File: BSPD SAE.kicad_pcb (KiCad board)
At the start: 2 copper layers, 70 x 70 mm, 66 parts, among them J1 430450412, J2 436500215, K1 G5Q-1A-EU DC12, Q1 MMBT3904, Q2 2N7002K, Q3 MMBT3904, U1 LTC6994xS6-2, U2 TPS7A2501DRVR, U3 TLV1824, U4 TLV1824

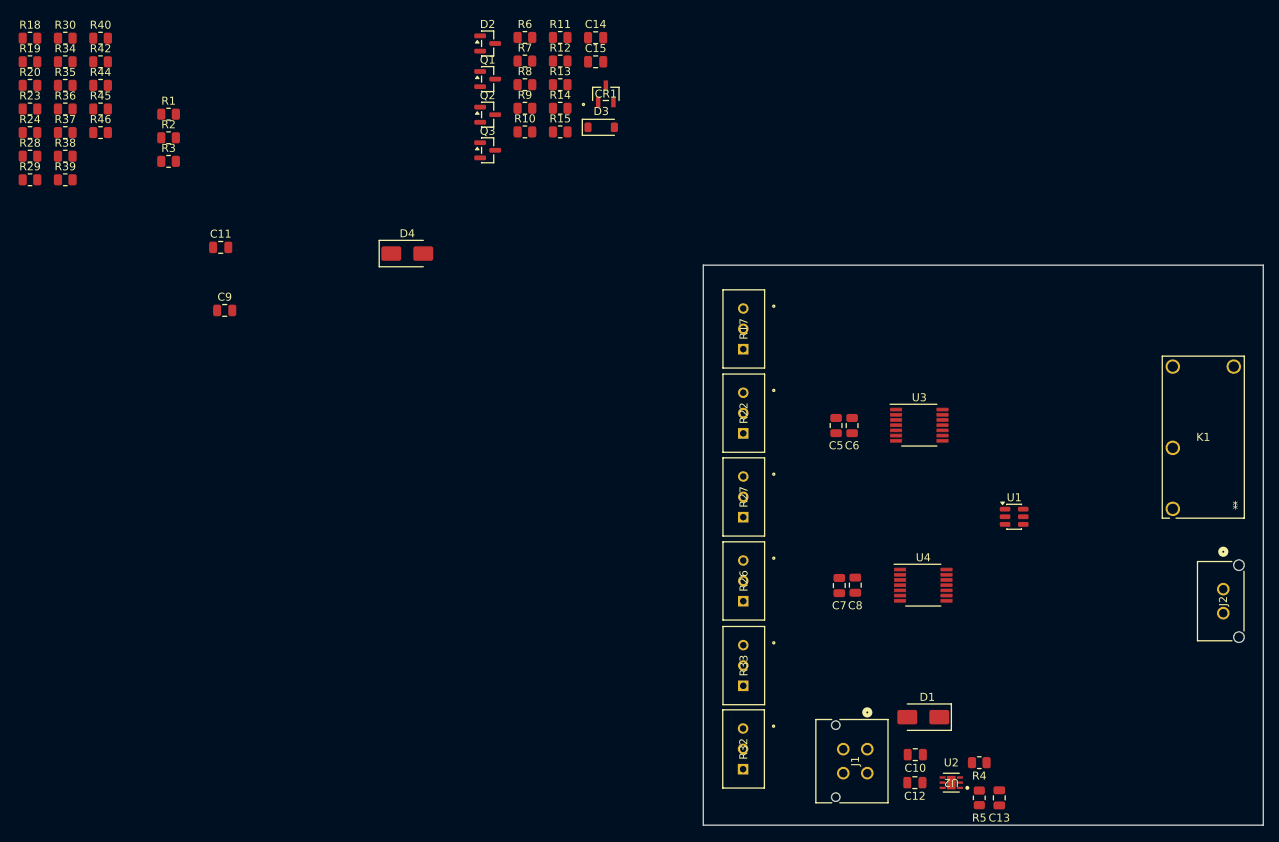
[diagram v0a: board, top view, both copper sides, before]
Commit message: autosave 2026-10-13 16:31:22
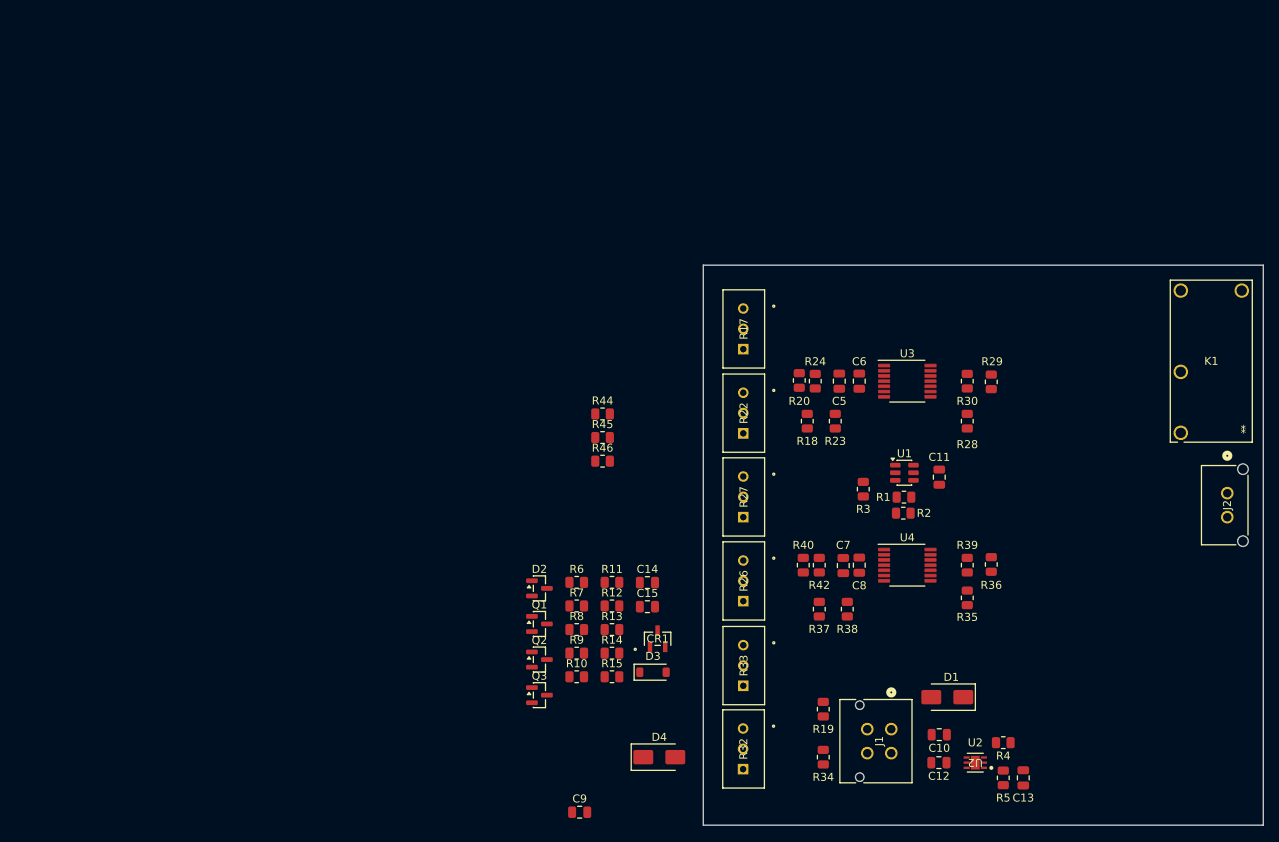
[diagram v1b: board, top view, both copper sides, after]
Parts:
- moved R35 129.7 mm to (153.0, 98.6), turned to 90 degrees
- moved R36 129.0 mm to (156.0, 94.4), turned to 90 degrees
- moved R34 128.6 mm to (135.0, 118.5), turned to 90 degrees
- moved R19 128.0 mm to (135.0, 112.5), turned to 90 degrees
- moved R29 122.8 mm to (156.0, 71.6), turned to 90 degrees
- moved R39 122.6 mm to (153.0, 94.5), turned to 90 degrees
- moved R28 121.8 mm to (153.0, 76.5), turned to 90 degrees
- moved R30 120.6 mm to (153.0, 71.5), turned to 90 degrees
- moved R38 113.0 mm to (138.0, 100.0), turned to 90 degrees
- moved R37 111.5 mm to (134.5, 100.0), turned to -90 degrees
- moved R40 109.8 mm to (132.5, 94.5), turned to 90 degrees
- moved R42 109.7 mm to (134.5, 94.5), turned to 90 degrees
- moved R18 108.3 mm to (133.0, 76.5), turned to 90 degrees
- moved R23 108.0 mm to (136.5, 76.5), turned to 90 degrees
- moved R1 103.6 mm to (145.1, 86.0)
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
